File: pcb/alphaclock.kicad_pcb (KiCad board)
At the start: 2 copper layers, 25.7 x 34.4 mm, 3 parts, among them P1 CONN_01X08, P2 CONN_01X08

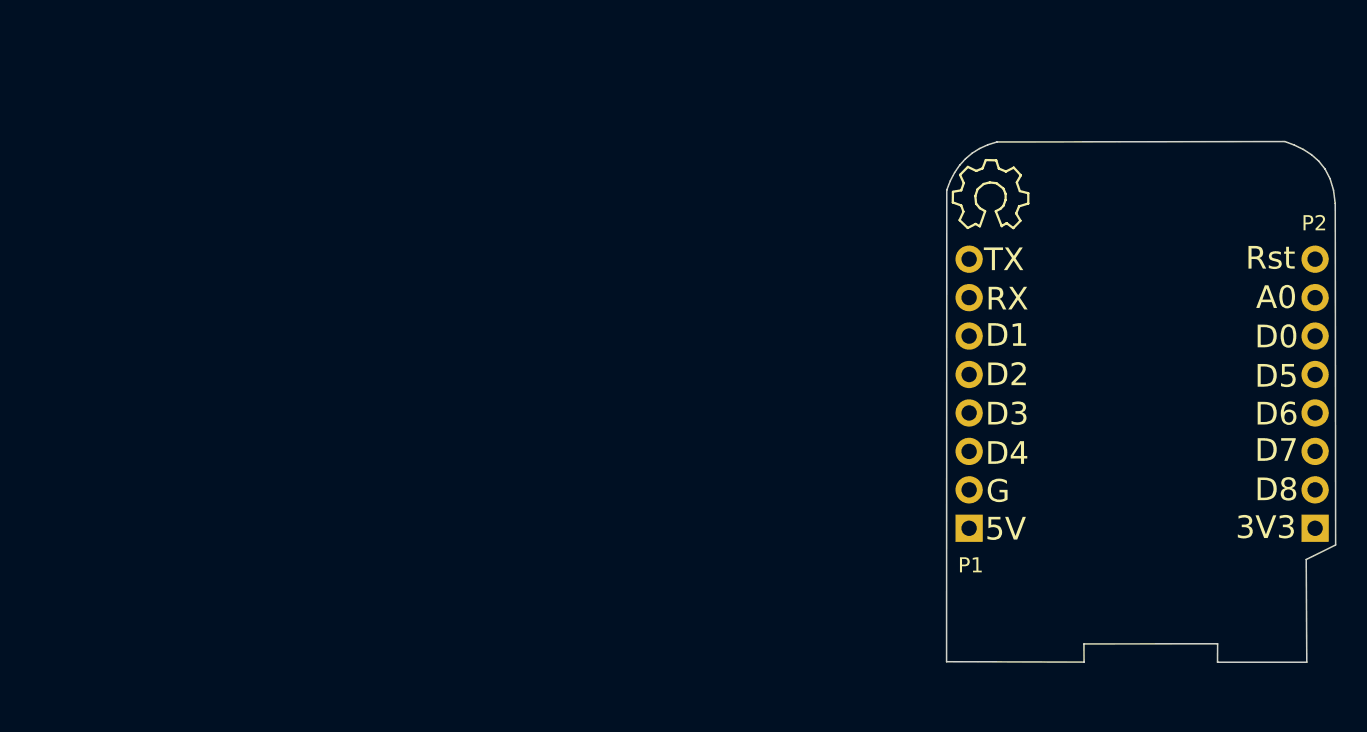
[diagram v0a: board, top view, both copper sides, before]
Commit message: Complete routing
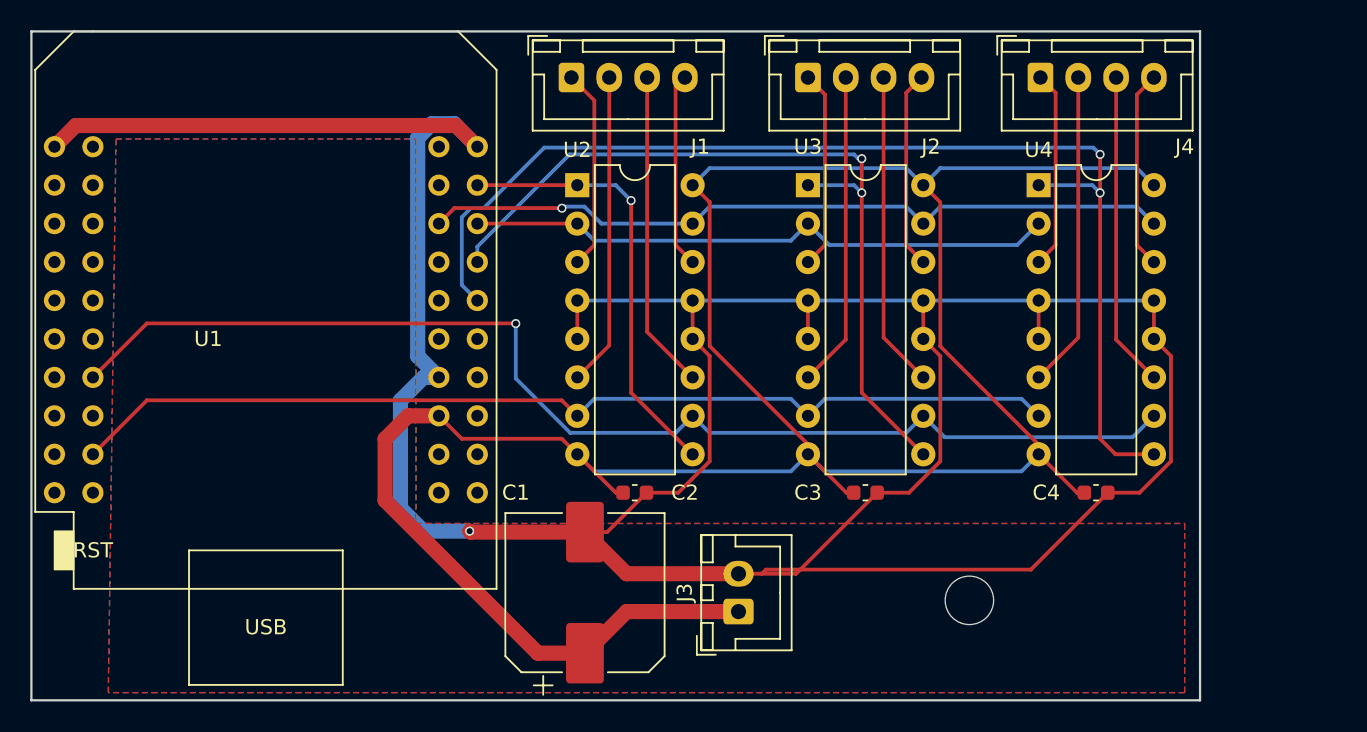
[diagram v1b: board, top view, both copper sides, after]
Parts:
- removed ?: OSHW, D1_mini:OSHW
- removed P1, P2: CONN_01X08, D1_mini:D1_mini_Pin_Header
- added C1: 100u, Capacitor_SMD:CP_Elec_10x10, F.Cu at (102.1, 108.2)
- added C2: 100n, Capacitor_SMD:C_0603_1608Metric, F.Cu at (105.4, 101.6)
- added C3: 100n, Capacitor_SMD:C_0603_1608Metric, F.Cu at (120.6, 101.6)
- added C4: 100n, Capacitor_SMD:C_0603_1608Metric, F.Cu at (135.9, 101.6)
- added H1: MountingHole, MountingHole:MountingHole_3.2mm_M3, F.Cu at (127.5, 108.7)
- added J1: Conn_01x04, Connector_JST:JST_XH_B4B-XH-A_1x04_P2.50mm_Vertical, F.Cu at (101.2, 74.2)
- added J2: Conn_01x04, Connector_JST:JST_XH_B4B-XH-A_1x04_P2.50mm_Vertical, F.Cu at (116.8, 74.2)
- added J3: Conn_01x02, Connector_JST:JST_XH_B2B-XH-A_1x02_P2.50mm_Vertical, F.Cu at (112.3, 109.5)
- added J4: Conn_01x04, Connector_JST:JST_XH_B4B-XH-A_1x04_P2.50mm_Vertical, F.Cu at (132.2, 74.2)
- added U1: mini_esp32, ESP32_mini:ESP32_mini, F.Cu at (81.0, 90.2)
- added U2: L293D, Package_DIP:DIP-16_W7.62mm, F.Cu at (101.6, 81.3)
- added U3: L293D, Package_DIP:DIP-16_W7.62mm, F.Cu at (116.8, 81.3)
- added U4: L293D, Package_DIP:DIP-16_W7.62mm, F.Cu at (132.1, 81.3)
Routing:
- net GND: track 0.00 -> 220.6 mm, vias 0 -> 1
- net +5V: track 0.00 -> 165.9 mm
- net 3A: track 0.00 -> 79.3 mm, vias 0 -> 1
- net EN3: track 0.00 -> 77.2 mm, vias 0 -> 2
- net 2A: track 0.00 -> 66.3 mm
- net EN2: track 0.00 -> 54.0 mm, vias 0 -> 2
- net 4A: track 0.00 -> 50.1 mm, vias 0 -> 1
- net 1A: track 0.00 -> 39.2 mm
- net Net-(U1-IO_27): track 0.00 -> 29.0 mm, vias 0 -> 1
- net Net-(J1-Pin_3): track 0.00 -> 21.1 mm
- net Net-(J2-Pin_3): track 0.00 -> 20.9 mm
- net Net-(J4-Pin_2): track 0.00 -> 20.9 mm
- net Net-(J4-Pin_3): track 0.00 -> 20.8 mm
- net Net-(J2-Pin_2): track 0.00 -> 20.8 mm
- net Net-(J1-Pin_2): track 0.00 -> 20.7 mm
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- added copper zone on B.Cu, net GND
- added copper zone on F.Cu, net GND
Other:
- board size 25.7 x 34.4 mm -> 77.2 x 44.2 mm
- net class Default removed
- board text removed: "3V3"
- board text removed: "5V"
- board text removed: "A0"
- board text removed: "D0"
- board text removed: "D1"
- board text removed: "D2"
- board text removed: "D3"
- board text removed: "D4"
- board text removed: "D5"
- board text removed: "D6"
- board text removed: "D7"
- board text removed: "D8"
- board text removed: "G"
- board text removed: "RX"
- board text removed: "Rst"
- board text removed: "TX"

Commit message: Order.
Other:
- rule pad_to_mask_clearance: 0.2 -> 0
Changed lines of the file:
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@@
 	)
 	(setup
-		(pad_to_mask_clearance 0.2)
+		(pad_to_mask_clearance 0)
 		(allow_soldermask_bridges_in_footprints no)
 		(tenting front back)
 		(pcbplotparams
-			(layerselection 0x00000000_00000000_00000000_000000a5)
+			(layerselection 0x00000000_00000000_55555555_575555ff)
 			(plot_on_all_layers_selection 0x00000000_00000000_00000000_00000000)
 			(disableapertmacros no)
@@
 			(outputformat 1)
 			(mirror no)
-			(drillshape 1)
+			(drillshape 0)
 			(scaleselection 1)
-			(outputdirectory "")
+			(outputdirectory "gerber")
 		)
 	)
